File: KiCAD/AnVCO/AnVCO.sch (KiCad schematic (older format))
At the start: 17 parts, among them J1 CV, J2 SW_WaveForm, J3 WAVE_OUT, J4 ERK_PWR, J5 SQR_OUT

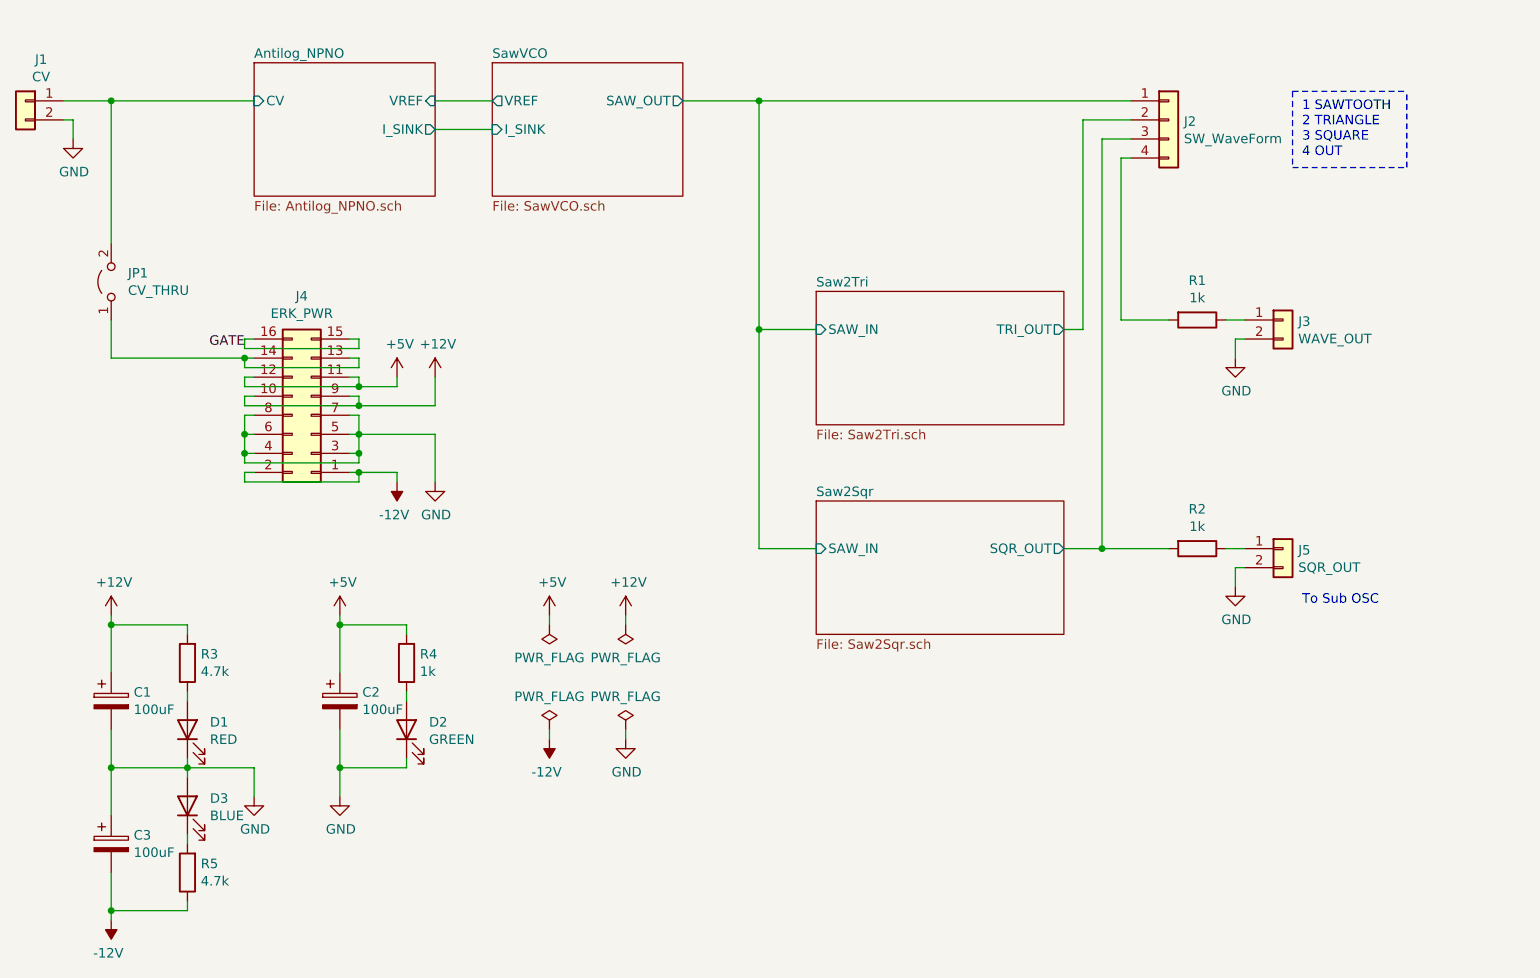
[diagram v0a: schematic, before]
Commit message: Before wiring
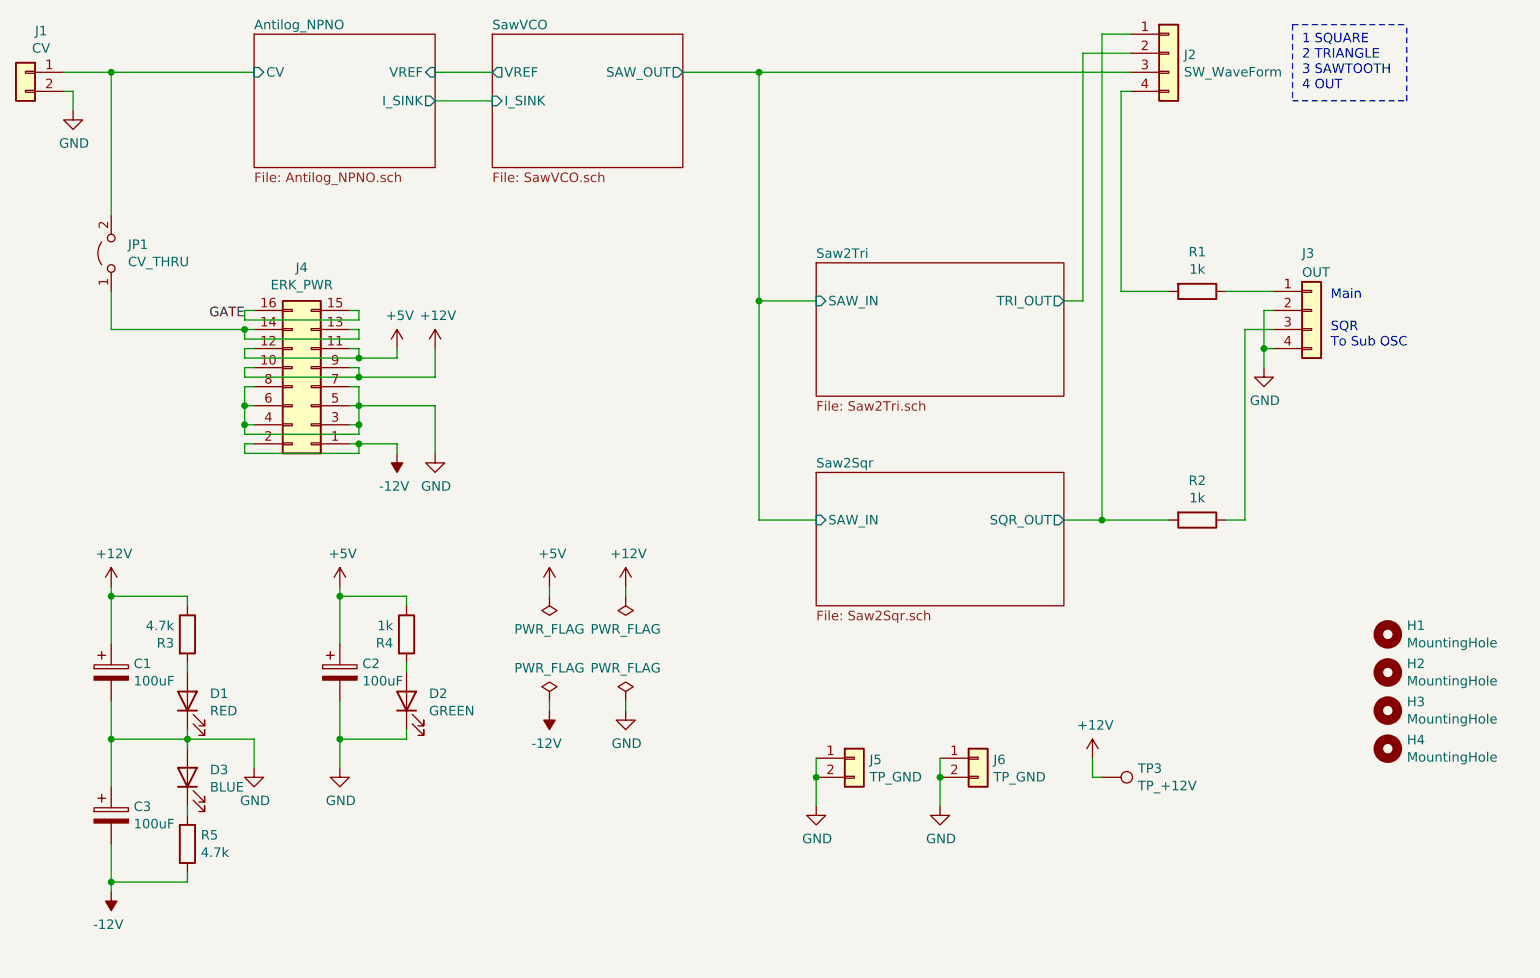
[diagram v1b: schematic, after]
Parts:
- removed J3: WAVE_OUT, Connector_JST:JST_XH_B2B-XH-A_1x02_P2.50mm_Vertical, symbol Connector_Generic:Conn_01x02
- added H1, H2, H3, H4: MountingHole, MountingHole:MountingHole_3.2mm_M3, symbol Mechanical:MountingHole
- added J3: OUT, Connector_JST:JST_XH_B4B-XH-A_1x04_P2.50mm_Vertical, symbol Connector_Generic:Conn_01x04
- added J6: TP_GND, Connector_PinHeader_2.54mm:PinHeader_1x02_P2.54mm_Vertical, symbol Connector_Generic:Conn_01x02
- added TP3: TP_+12V, TestPoint:TestPoint_THTPad_D2.0mm_Drill1.0mm, symbol Connector:TestPoint
- J5: value SQR_OUT -> TP_GND; footprint Connector_JST:JST_XH_B2B-XH-A_1x02_P2.50mm_Vertical -> Connector_PinHeader_2.54mm:PinHeader_1x02_P2.54mm_Vertical
- R3, R4, R5: footprint Resistor_THT:R_Axial_DIN0207_L6.3mm_D2.5mm_P10.16mm_Horizontal -> Resistor_THT:R_Axial_DIN0207_L6.3mm_D2.5mm_P2.54mm_Vertical
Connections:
- net +12V: now also R3.1, TP3.1; no longer R3.2
- net +5V: now also R4.1; no longer R4.2
- net GND: now also J5.1 (Pin_1), J3.2 (Pin_2), J3.4 (Pin_4), J6.1 (Pin_1), J6.2 (Pin_2)
- net Saw2Sqr/SAW_IN: now also J2.3 (Pin_3); no longer J2.1 (Pin_1)
- net Saw2Sqr/SQR_OUT: now also J2.1 (Pin_1); no longer J2.3 (Pin_3)
- net at R1.1: now also J3.1 (Pin_1)
- net at D1.2 (A): now also R3.2; no longer R3.1
- net at D2.2 (A): now also R4.2; no longer R4.1
- net at R2.1: now also J3.3 (Pin_3); no longer J5.1 (Pin_1)
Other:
- note added: "1 SQUARE\n2 TRIANGLE\n3 SAWTOOTH\n4 OUT"
- note added: "Main"
- note added: "SQR\nTo Sub OSC"
- note removed: "1 SAWTOOTH\n2 TRIANGLE\n3 SQUARE\n4 OUT"
- note removed: "To Sub OSC"
- moved on the sheet: C1, C2, C3, D1, D2, D3, J1, J2, J4, JP1, R1, R2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
